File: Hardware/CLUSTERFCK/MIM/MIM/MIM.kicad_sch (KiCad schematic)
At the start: 22 parts, among them J1 Conn_02x20_Counter_Clockwise, J2 Conn_02x20_Counter_Clockwise, U1 74LS00, U10 74LS245, U2 INTEL2716, U3 INTEL2716, U4 74LS161, U5 INTEL2716, U6 74LS245, U7 74LS245, U8 74LS245, U9 74LS245

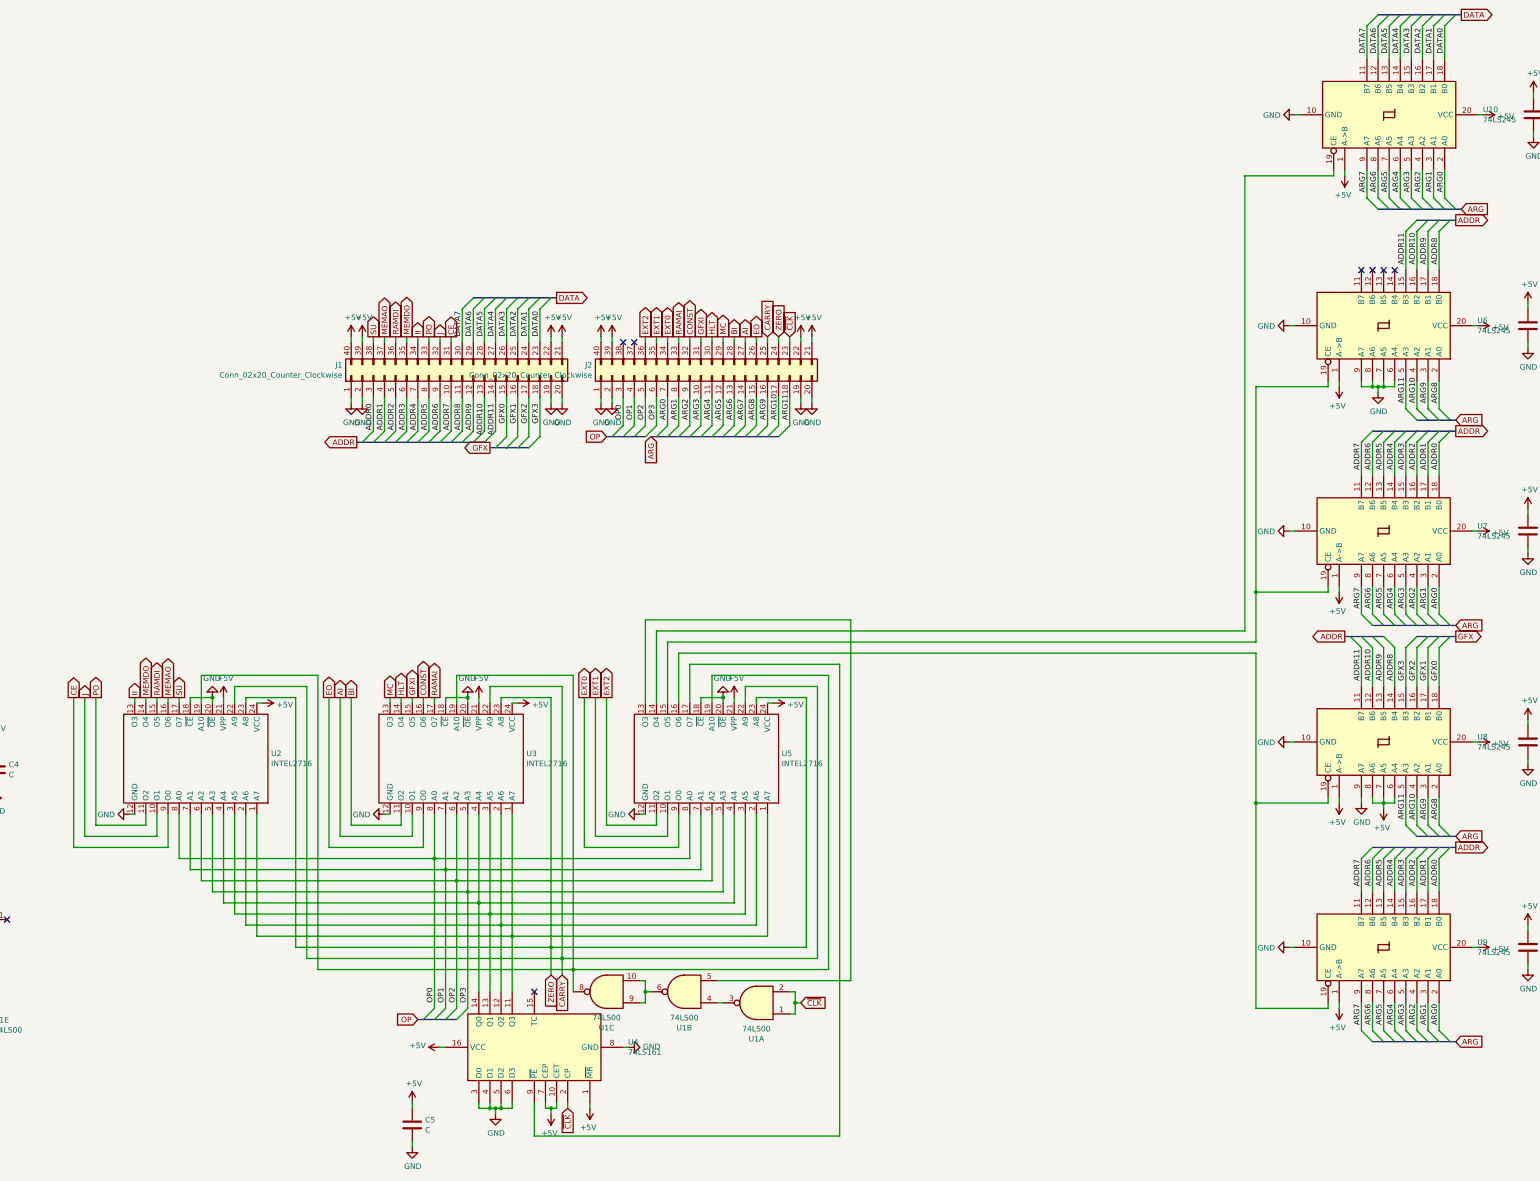
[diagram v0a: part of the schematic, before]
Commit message: 0065 | 24h | ADDR & DATA & PLACEHOLDER etc
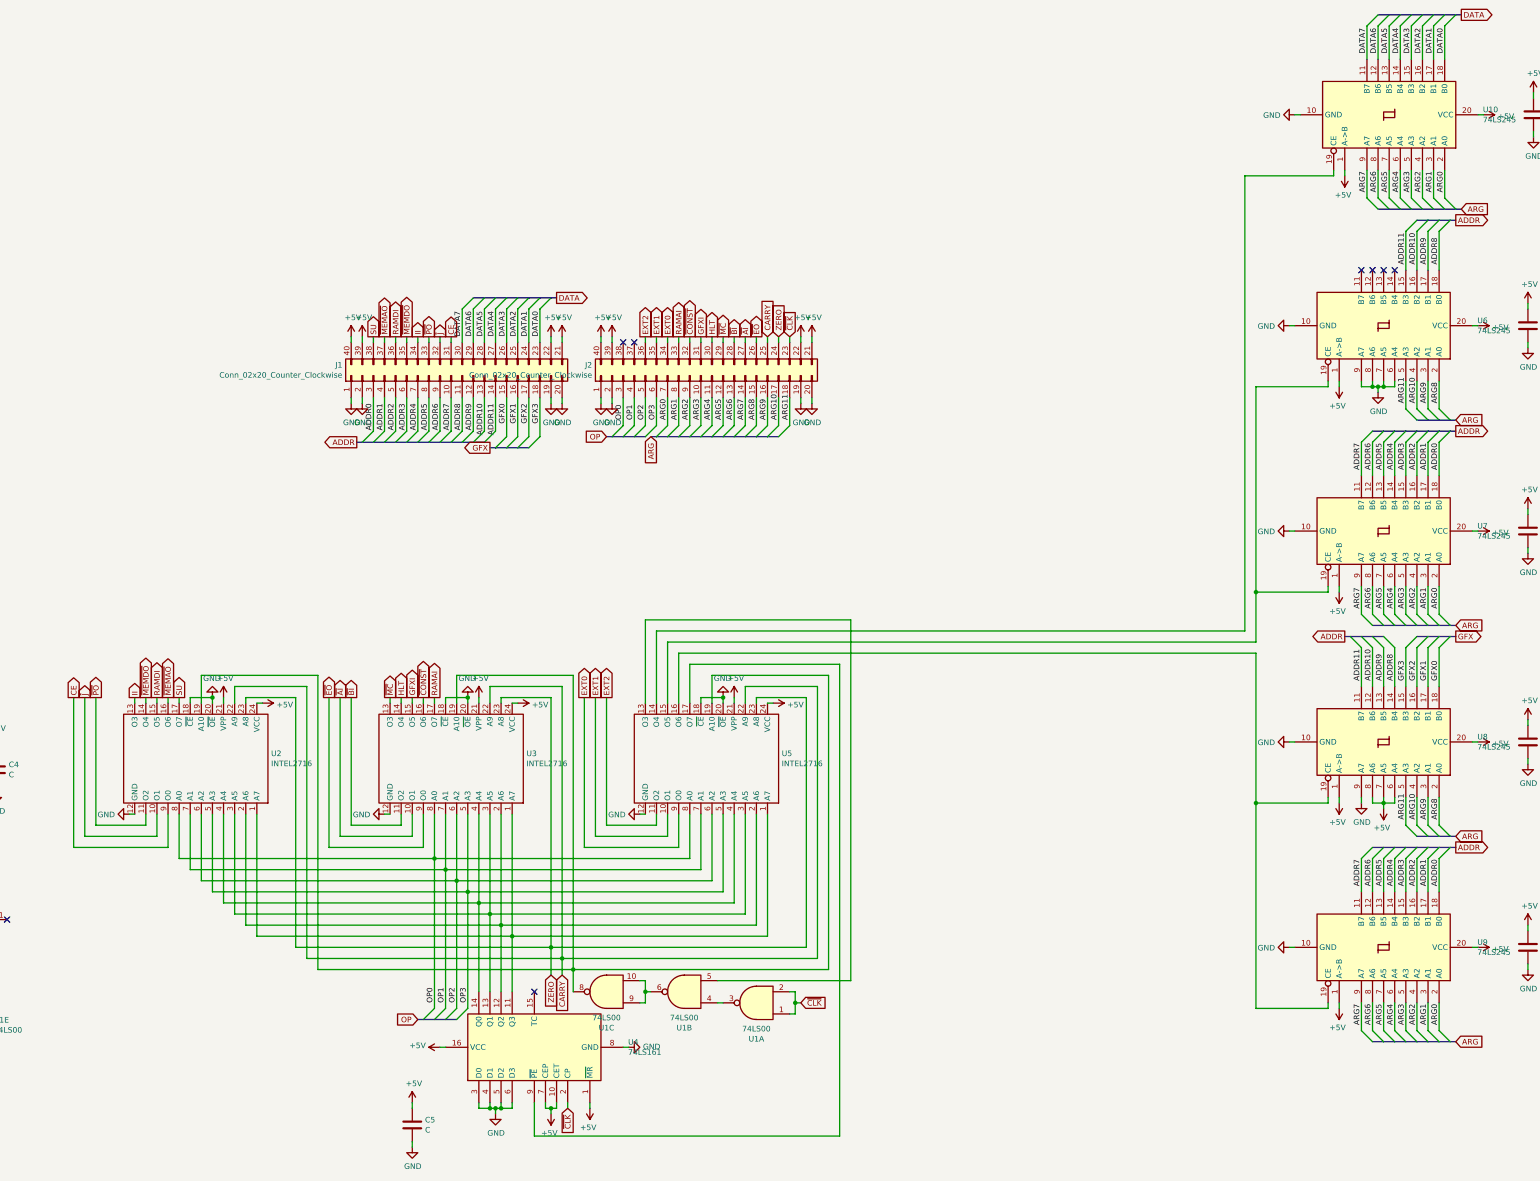
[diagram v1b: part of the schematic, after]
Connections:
- net AI renamed ~AI
- net BI renamed ~BI
- net CONST renamed ~CONST
- net EO renamed ~EO
- net J renamed ~J
- net MC renamed ~MC
- net MEMAO renamed ~MEMAO
- net MEMDO renamed ~MEMDO
- net PO renamed ~PO
